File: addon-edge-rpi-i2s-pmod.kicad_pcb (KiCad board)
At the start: 2 copper layers, 100 x 72 mm, 38 parts, among them J1 PMOD1, J10 Conn_01x02, J11 Conn_01x01, J2 PMOD2, J3 PMOD3, J4 Conn_01x06, J5 Conn_01x06, J6 Conn_02x04_Top_Bottom, J7 Conn_01x03, J8 Conn_01x04, J9 Conn_01x05

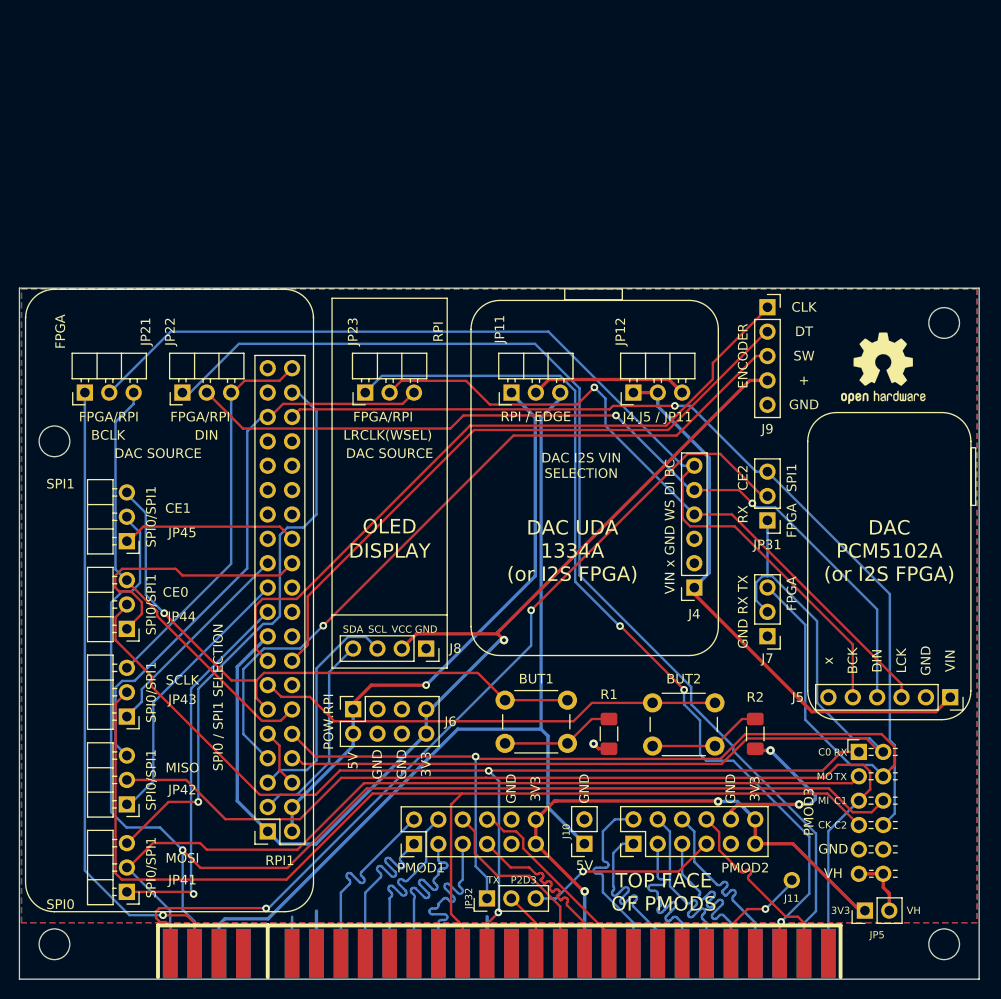
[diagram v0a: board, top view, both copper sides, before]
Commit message: v0.50 major changes
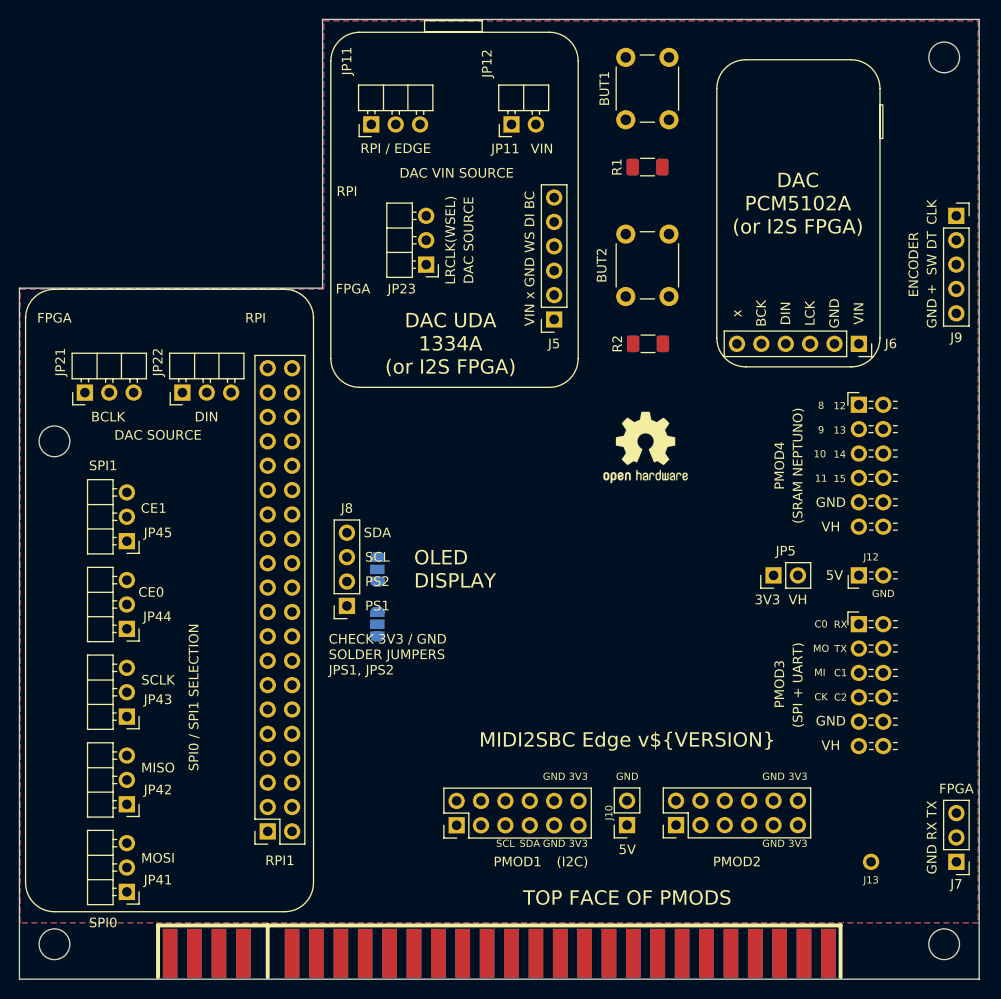
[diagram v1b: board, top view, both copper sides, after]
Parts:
- removed the J6 at (143.5, 116.8)
- removed JP31, JP32: Conn_01x03, Connector_PinHeader_2.54mm:PinHeader_1x03_P2.54mm_Vertical
- added J12: Conn_01x02, Connector_PinSocket_2.54mm:PinSocket_2x01_P2.54mm_Horizontal, F.Cu at (196.2, 102.9)
- added J4: PMOD4, gomaDOSzero:PMOD_Female_Horizontal_2, F.Cu at (196.2, 97.8)
- added JPS1: SolderJumper_3_Open, Jumper:SolderJumper-3_P1.3mm_Open_RoundedPad1.0x1.5mm_NumberLabels, B.Cu at (146.1, 108.0)
- added JPS2: SolderJumper_3_Open, Jumper:SolderJumper-3_P1.3mm_Open_RoundedPad1.0x1.5mm_NumberLabels, B.Cu at (146.1, 102.2)
- J8: footprint gomaDOSzero:OLED_091_DISPLAY -> gomaDOSzero:I2C_DISPLAY_MULTI2
- JP12: value Conn_01x03 -> Conn_01x02; footprint Connector_PinHeader_2.54mm:PinHeader_1x03_P2.54mm_Horizontal -> Connector_PinHeader_2.54mm:PinHeader_1x02_P2.54mm_Horizontal
- moved LO4 85.4 mm to (127.6, 132.7)
- moved BUT1 72.3 mm to (176.4, 48.9), turned to -90 degrees
- moved R1 59.2 mm to (174.2, 60.3), turned to 180 degrees
- moved BUT2 53.6 mm to (176.4, 67.3), turned to -90 degrees
- moved LO3 43.8 mm to (191.8, 61.0)
- moved R2 42.1 mm to (174.2, 78.7), turned to 180 degrees
- moved J6 37.0 mm to (196.2, 78.7), turned to -90 degrees
- moved JP5 36.2 mm to (187.3, 102.9)
- moved JP11 31.5 mm to (145.4, 55.9)
- moved J5 31.5 mm to (164.5, 76.2)
- moved JP12 30.7 mm to (160.0, 55.9)
- moved J7 30.7 mm to (206.4, 132.7)
- moved H1 27.7 mm to (205.1, 48.9)
- moved LO2 26.1 mm to (174.0, 89.5)
- moved J9 21.9 mm to (206.4, 65.4)
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- renumbered J11 to J13, J4 to J5, J5 to J6, REF** to LO1, OH2 to LO2, OH1 to LO3, ESD1 to LO4
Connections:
- net Net-(J3-Pad12) renamed /VH_PMOD
- EDGE1 pad A12: /A12_PMOD1_D2 -> /A12_PMOD1_D6
- EDGE1 pad A20: /A20_PMOD2_D4 -> /A20_PMOD2_D5
- EDGE1 pad A21: /A21_PMOD2_D0 -> /A21_PMOD2_D1
- EDGE1 pad A22: /A22_PMOD2_D1 -> /A22_PMOD2_D6
- EDGE1 pad A23: /A23_PMOD2_D5 -> /A23_PMOD2_D2
- EDGE1 pad A24: /A24_PMOD2_D2 -> /A24_PMOD2_D7
- EDGE1 pad A25: /A25_PMOD2_D6 -> /A25_PMOD2_D3
- EDGE1 pad B1: /B1_CE2_UART_RX -> /B1_UART_RX
- EDGE1 pad B10: unconnected-(EDGE1-PadB10) -> /B10_SRAMDQ13
- EDGE1 pad B11: unconnected-(EDGE1-PadB11) -> /B11_SRAMDQ11
- EDGE1 pad B12: unconnected-(EDGE1-PadB12) -> /B12_SRAMDQ12
- EDGE1 pad B15: unconnected-(EDGE1-PadB15) -> /B15_SCL_PM1_D2
- EDGE1 pad B16: /B16_PMOD_UARTX_MIDI -> /B16_UART_TX_MIDI
- EDGE1 pad B17: /B17_PMOD1_D6 -> /B17_PMOD1_D7
- EDGE1 pad B18: /B18_PMOD1_D3 -> /B18_PMOD2_D4
- EDGE1 pad B19: /B19_PMOD1_D7 -> /B19_PMOD2_D0
- EDGE1 pad B21: unconnected-(EDGE1-PadB21) -> /B21_SDA_PM1_D3
- EDGE1 pad B27: /B27_PMOD2_D7 -> /B27_SPI1CE2
- EDGE1 pad B3: unconnected-(EDGE1-PadB3) -> /B3_SRAMDQ15
- EDGE1 pad B6: unconnected-(EDGE1-PadB6) -> /B6_SRAMDQ8
- EDGE1 pad B7: unconnected-(EDGE1-PadB7) -> /B7_SRAMDQ9
- EDGE1 pad B8: unconnected-(EDGE1-PadB8) -> /B8_SRAMDQ10
- EDGE1 pad B9: unconnected-(EDGE1-PadB9) -> /B9_SRAMDQ14
- J1 pad 10: /B19_PMOD1_D7 -> /B17_PMOD1_D7
- J1 pad 3: /A12_PMOD1_D2 -> /B15_SCL_PM1_D2
- J1 pad 4: /B18_PMOD1_D3 -> /B21_SDA_PM1_D3
- J1 pad 9: /B17_PMOD1_D6 -> /A12_PMOD1_D6
- J2 pad 1: /A21_PMOD2_D0 -> /B19_PMOD2_D0
- J2 pad 10: /B27_PMOD2_D7 -> /A24_PMOD2_D7
- J2 pad 2: /A22_PMOD2_D1 -> /A21_PMOD2_D1
- J2 pad 3: /A24_PMOD2_D2 -> /A23_PMOD2_D2
- J2 pad 4: /B16_PMOD2_D3 -> /A25_PMOD2_D3
- J2 pad 7: /A20_PMOD2_D4 -> /B18_PMOD2_D4
- J2 pad 8: /A23_PMOD2_D5 -> /A20_PMOD2_D5
- J2 pad 9: /A25_PMOD2_D6 -> /A22_PMOD2_D6
- J3 pad 10: /B1_SPI1_CE2 -> /B27_SPI1CE2
- J8 pad 1: GND -> /DISPLAY_PS1
- J8 pad 2: 3V3pi -> /DISPLAY_PS2
- JP12 pad 1: VIN -> /JP11_Vout
- RPI1 pad 36: /B1_SPI1_CE2 -> /B27_SPI1CE2
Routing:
- net /A2_CE1: track 132.3 -> 0.00 mm, vias 1 -> 0
- net /B13_SCLK_DABD: track 119.8 -> 0.00 mm
- net /A27_DIN_I2S: track 115.0 -> 0.00 mm
- net /B14_CE0_CLKBD: track 110.9 -> 0.00 mm, vias 2 -> 0
- net /B16_UART_TX_MIDI: track 110.3 -> 0.00 mm, vias 1 -> 0
- net 3V3pi: track 109.1 -> 0.00 mm, vias 1 -> 0
- net /DAC_BCLK_I2S: track 104.1 -> 0.00 mm
- net /A28_MISO_WSBD: track 102.5 -> 0.00 mm
- net /B1_UART_RX: track 98.9 -> 0.00 mm
- net /B1_SPI1_CE2: track 95.7 -> 0.00 mm, vias 1 -> 0
- net /B26_WSEL_LRCLK_I2S: track 94.9 -> 0.00 mm, vias 3 -> 0
- net +5V: track 94.7 -> 0.00 mm
- net /B1_CE2_UART_RX: track 92.8 -> 0.00 mm, vias 2 -> 0
- net /A1_MOSI: track 91.6 -> 0.00 mm
- net /DAC_DIN_I2S: track 89.5 -> 0.00 mm, vias 2 -> 0
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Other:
- board size 100 x 72 mm -> 100 x 100 mm
- board text added: "(I2C)"
- board text added: "(SPI + UART)"
- board text added: "(SRAM NEPTUNO)"
- board text added: "10"
- board text added: "11"
- board text added: "12"
- board text added: "13"
- board text added: "14"
- board text added: "15"
- board text added: "8"
- board text added: "9"
- board text added: "CHECK 3V3 / GND SOLDER JUMPERS JPS1, JPS2"
- board text added: "DAC VIN SOURCE"
- board text added: "JP11"
- board text added: "MIDI2SBC Edge v${VERSION}"
- board text added: "OLED DISPLAY"
- board text added: "PS1"
- board text added: "PS2"
- board text added: "SCL"
- board text added: "SDA"
- board text removed: "CE2"
- board text removed: "DAC I2S VIN SELECTION"
- board text removed: "FPGA/RPI"
- board text removed: "J4.J5 / JP11"
- board text removed: "P2D3"
- board text removed: "POW.RPI"
- board text removed: "SPI0/SPI1"
